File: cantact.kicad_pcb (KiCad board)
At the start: 2 copper layers, 36 x 16.4 mm, 38 parts, among them J1 USB_C_Receptacle_USB2.0, J2 Conn_01x04, J3 Conn_01x06, SW1 SW_SPST, SW2 SW_DPDT_x2, U1 NJM2871, U2 STM32F042C6Ux, U3 MCP2562-E-MF, Y1 Resonator

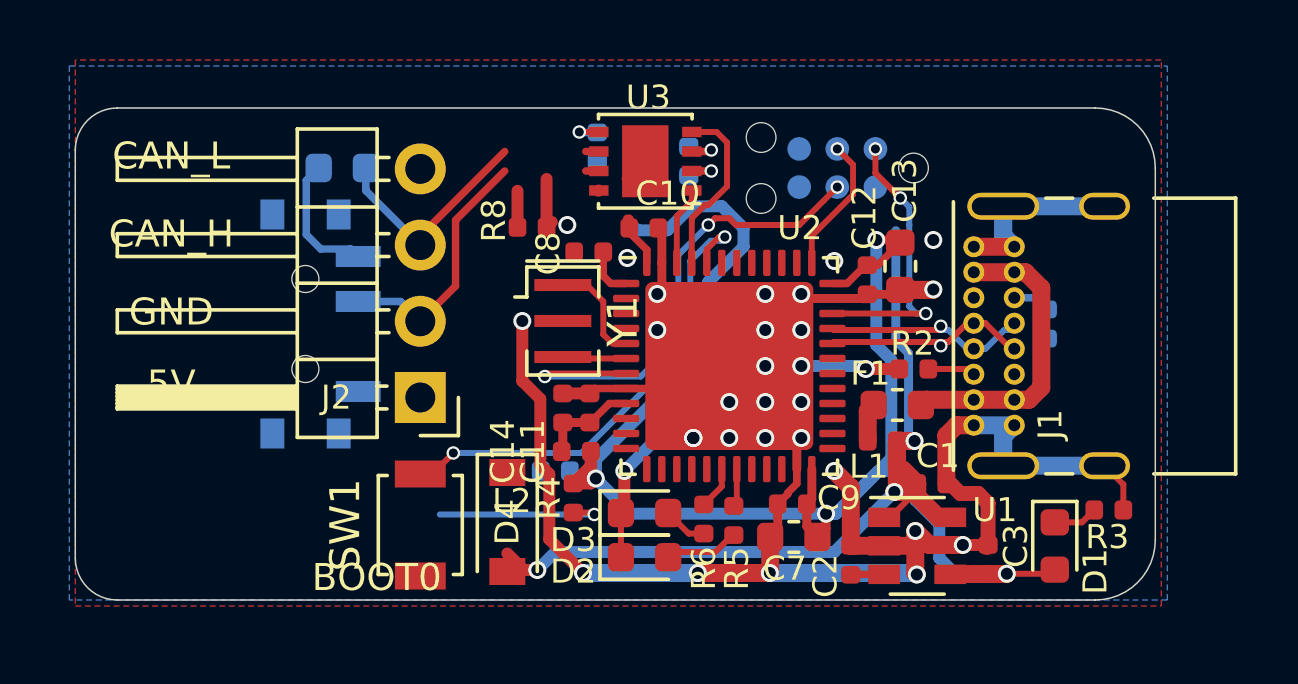
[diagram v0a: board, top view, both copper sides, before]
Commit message: 電源LEDの配置いじった
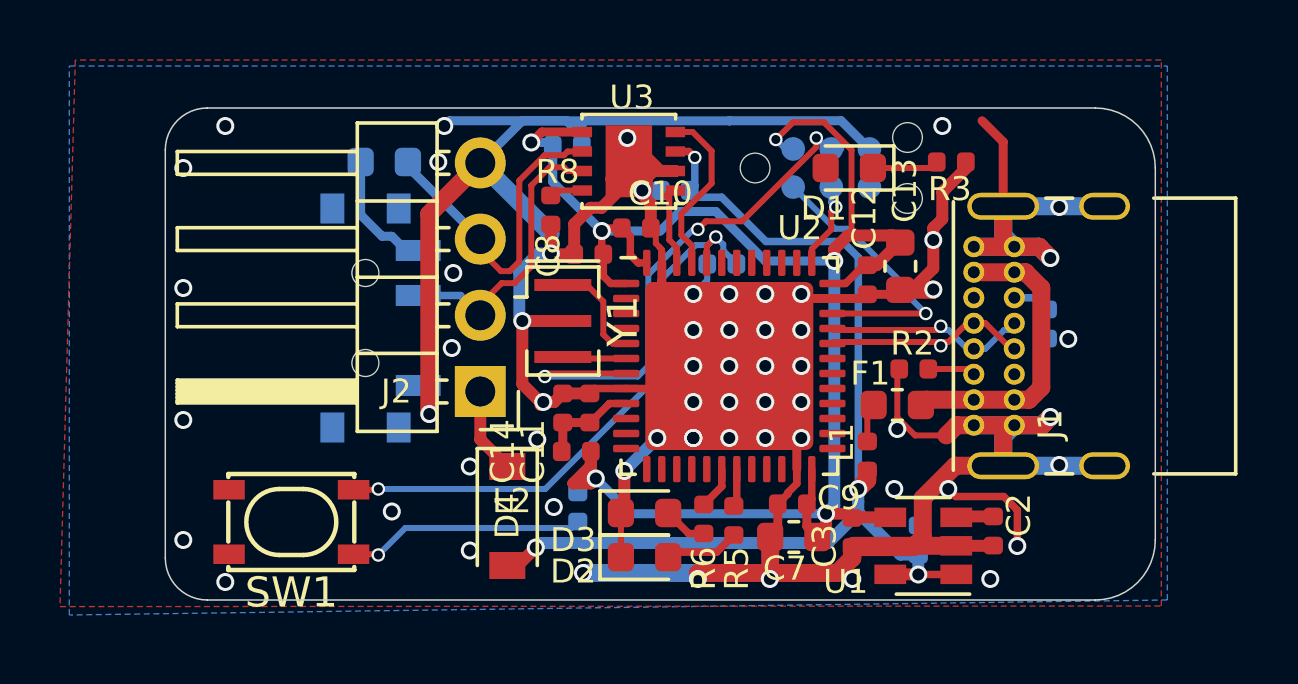
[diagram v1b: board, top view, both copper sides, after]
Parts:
- C1, R4: moved to B.Cu
- SW1: value SW_SPST -> SKRPACE010; footprint Button_Switch_SMD:SW_SPST_B3U-1000P -> Button_Switch_SMD_my:ALPS_SKRPAxE010
- moved D1 14.3 mm to (159.8, 111.4), turned to 180 degrees
- moved R3 12.7 mm to (163.2, 111.2)
- moved R7 8.86 mm to (155.6, 114.6)
- moved C2 4.85 mm to (164.6, 123.5), turned to 270 degrees
- moved C3 4.61 mm to (159.9, 123.5), turned to 270 degrees
- moved SW1 4.30 mm to (141.2, 123.2), turned to 180 degrees
- moved J2 2.01 mm to (147.5, 118.8)
- moved SW2 2.01 mm to (144.0, 116.4)
- moved C1 1.93 mm to (162.1, 123.8), turned to 90 degrees
- moved R9 1.41 mm to (144.3, 111.2)
- moved C16 1.07 mm to (154.0, 112.2), turned to 180 degrees
- moved C15 1.00 mm to (150.4, 110.7), turned to 0 degrees
- moved R8 0.85 mm to (149.8, 112.8), turned to 270 degrees
- moved L1 0.71 mm to (160.4, 121.0), turned to 270 degrees
- moved U3 0.55 mm to (152.4, 111.2)
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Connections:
- net Net-(J2-Pad2) renamed /CAN_+
- net Net-(J2-Pad3) renamed /CAN_-
- SW1 pad 2: Net-(R7-Pad1) -> (no net)
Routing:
- net GND: track 86.7 -> 151.4 mm, vias 30 -> 61
- net +5V: track 30.3 -> 35.8 mm
- net Net-(R7-Pad1): track 16.3 -> 19.7 mm
- net Net-(D4-Pad1): track 0.00 -> 2.87 mm
- net /CAN_-: track 8.04 -> 10.9 mm
- net Net-(R4-Pad2): track 5.88 -> 7.95 mm
- net +3V3: track 62.6 -> 60.8 mm, vias 7 -> 6
- net SWCLK: track 4.58 -> 2.92 mm
- net Net-(R5-Pad2): track 1.22 -> 2.49 mm
- net NRST: track 16.9 -> 18.0 mm
- net Net-(D1-Pad1): track 1.49 -> 2.21 mm
- net /CAN_+: track 8.95 -> 9.63 mm
- net SWDIO: track 9.48 -> 9.41 mm, vias 3 -> 1
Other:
- board size 36 x 16.4 mm -> 33 x 16.4 mm
- board text added: "+5V"
- board text added: "BOOT"
- board text added: "CAN"
- board text added: "Terminate"
- board text removed: "5V"
- board text removed: "BOOT0"
- board text removed: "SWCLK"
- board text removed: "Vtgt"
